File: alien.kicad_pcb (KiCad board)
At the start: 2 copper layers, 70 x 84 mm, 51 parts, among them Q1 2N3904, Q2 2N3904, Q3 2N5457, U1 LM324, X1 JD_CONN_01X01, X10 JD_CONN_01X01, X11 JD_CONN_01X01, X12 JD_CONN_01X02, X13 JD_CONN_01X02, X2 JD_CONN_01X01, X3 JD_CONN_01X01, X4 JD_CONN_01X01, X5 JD_CONN_01X01, X6 JD_CONN_01X01, X7 JD_CONN_01X01, X8 JD_CONN_01X01, X9 JD_CONN_01X01

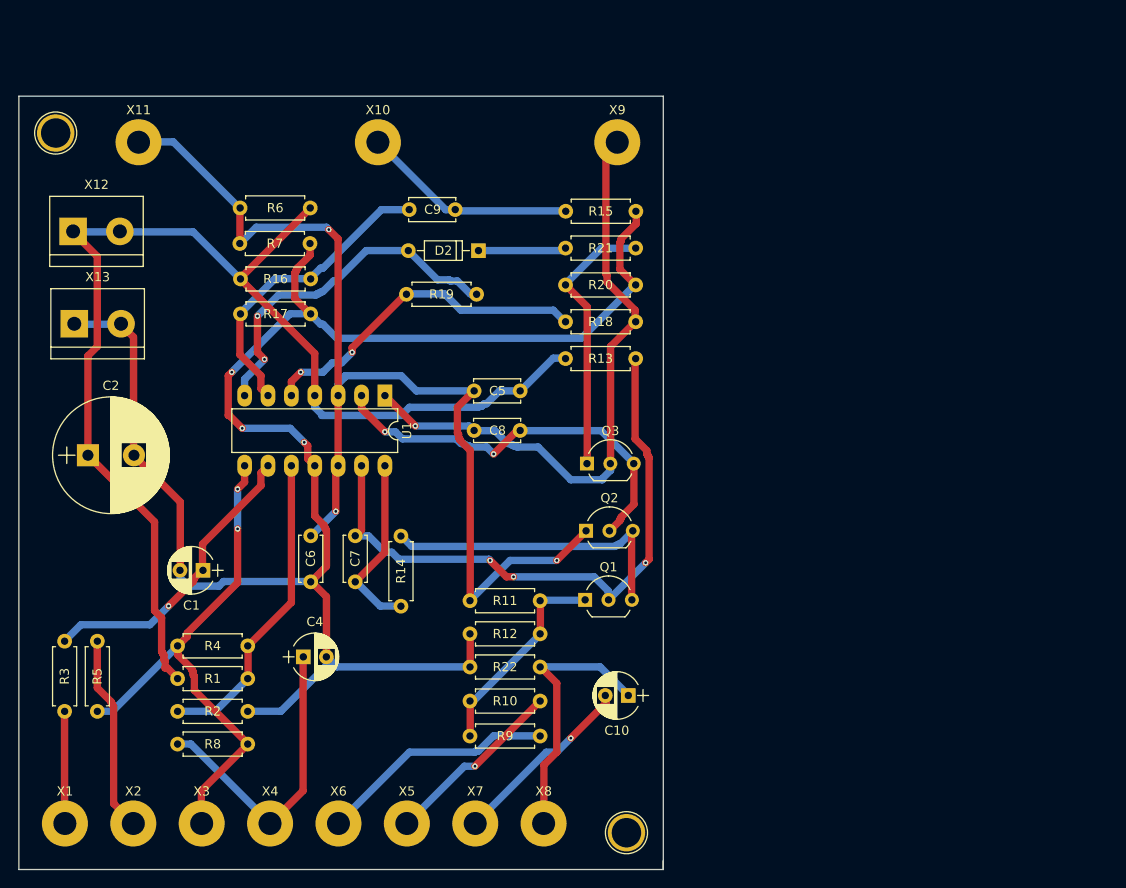
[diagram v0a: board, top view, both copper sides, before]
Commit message: amo que nos vamos
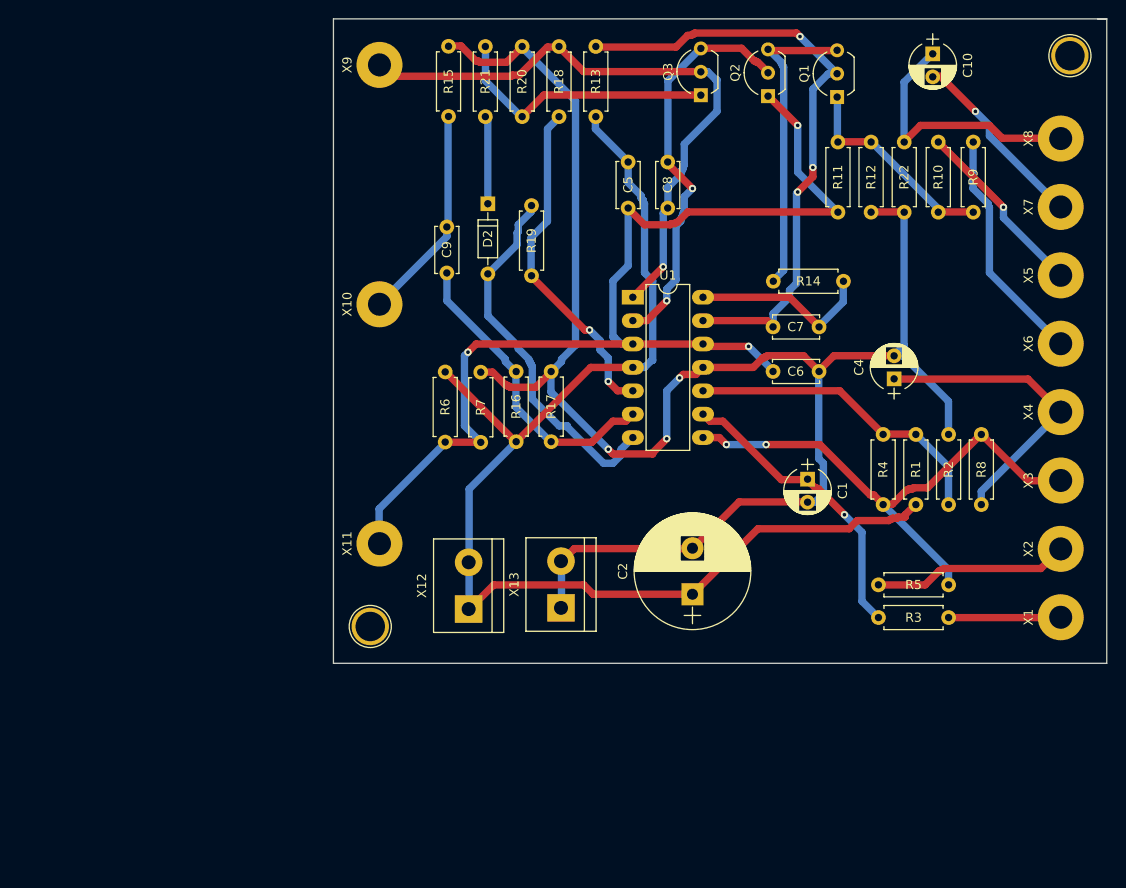
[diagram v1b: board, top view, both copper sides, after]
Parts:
- moved X1 110.5 mm to (185.2, 120.6), turned to 90 degrees
- moved X2 105.1 mm to (185.2, 113.2), turned to 90 degrees
- moved X3 100.5 mm to (185.2, 105.7), turned to 90 degrees
- moved REF** 97.2 mm to (186.2, 59.6), turned to 90 degrees
- moved X4 96.8 mm to (185.2, 98.3), turned to 90 degrees
- moved R3 96.6 mm to (173.0, 120.6), turned to 180 degrees
- moved X6 94.2 mm to (185.2, 90.9), turned to 90 degrees
- moved R5 93.5 mm to (173.0, 117.1), turned to 180 degrees
- moved X8 93.2 mm to (185.2, 68.6), turned to 90 degrees
- moved X5 92.7 mm to (185.2, 83.5), turned to 90 degrees
- moved X7 92.4 mm to (185.2, 76.0), turned to 90 degrees
- moved R8 91.1 mm to (176.5, 108.4), turned to 90 degrees
- moved R2 86.7 mm to (173.0, 108.4), turned to 90 degrees
- moved R1 82.4 mm to (169.4, 108.4), turned to 90 degrees
- moved R9 78.9 mm to (175.7, 76.6), turned to 90 degrees
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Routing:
- net Net-(D2-Pad2): track 38.6 -> 40.4 mm, vias 2 -> 0
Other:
- board size 70 x 84 mm -> 84 x 70 mm
- net class Default: via_dia 0.6 -> 0.8; via_drill 0.4 -> 0.5
- net class sinte: via_dia 0.6 -> 0.8; via_drill 0.4 -> 0.5
